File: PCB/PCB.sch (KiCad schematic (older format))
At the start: 17 parts, among them J1 PWM, J10 3V3, J11 I2C 1.1, J12 I2C 2.1, J13 PWM, J14 I2C 1.2, J15 I2C 2.2, J16 I2C 1.3, J17 I2C 2.3, J2 5V, J3 5V, J4 GND, J5 GND, J6 GND, J7 Raspberry_Pi_2_3, J8 GND, J9 3V3

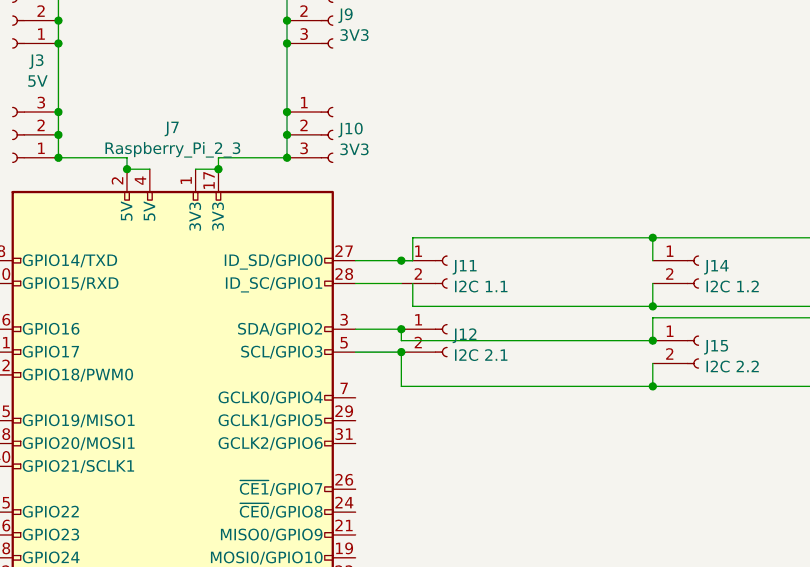
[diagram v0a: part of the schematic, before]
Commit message: Add gerber files
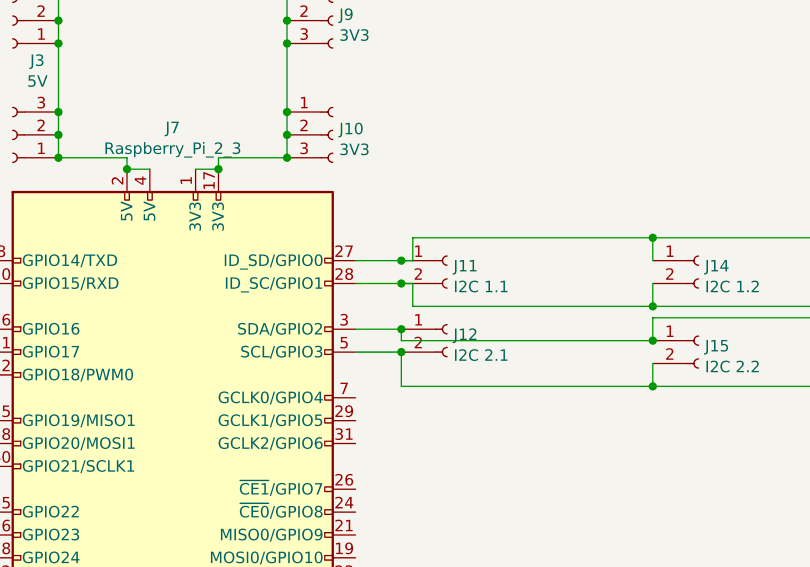
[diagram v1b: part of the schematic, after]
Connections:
- net at J11.2 (Pin_2), J7.28 (ID_SC/GPIO1): now also J14.2 (Pin_2), J16.2 (Pin_2)
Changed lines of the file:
@@
 	1    0    0    -1
 $EndComp
+Wire Wire Line
+	6000 2900 5950 2900
+Connection ~ 5950 2900
 $EndSCHEMATC
